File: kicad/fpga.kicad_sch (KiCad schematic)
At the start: 109 parts, among them Q4 BSS138LT1G, U1 XC7A100T-2FGG676I, X4 50MHz CMOS

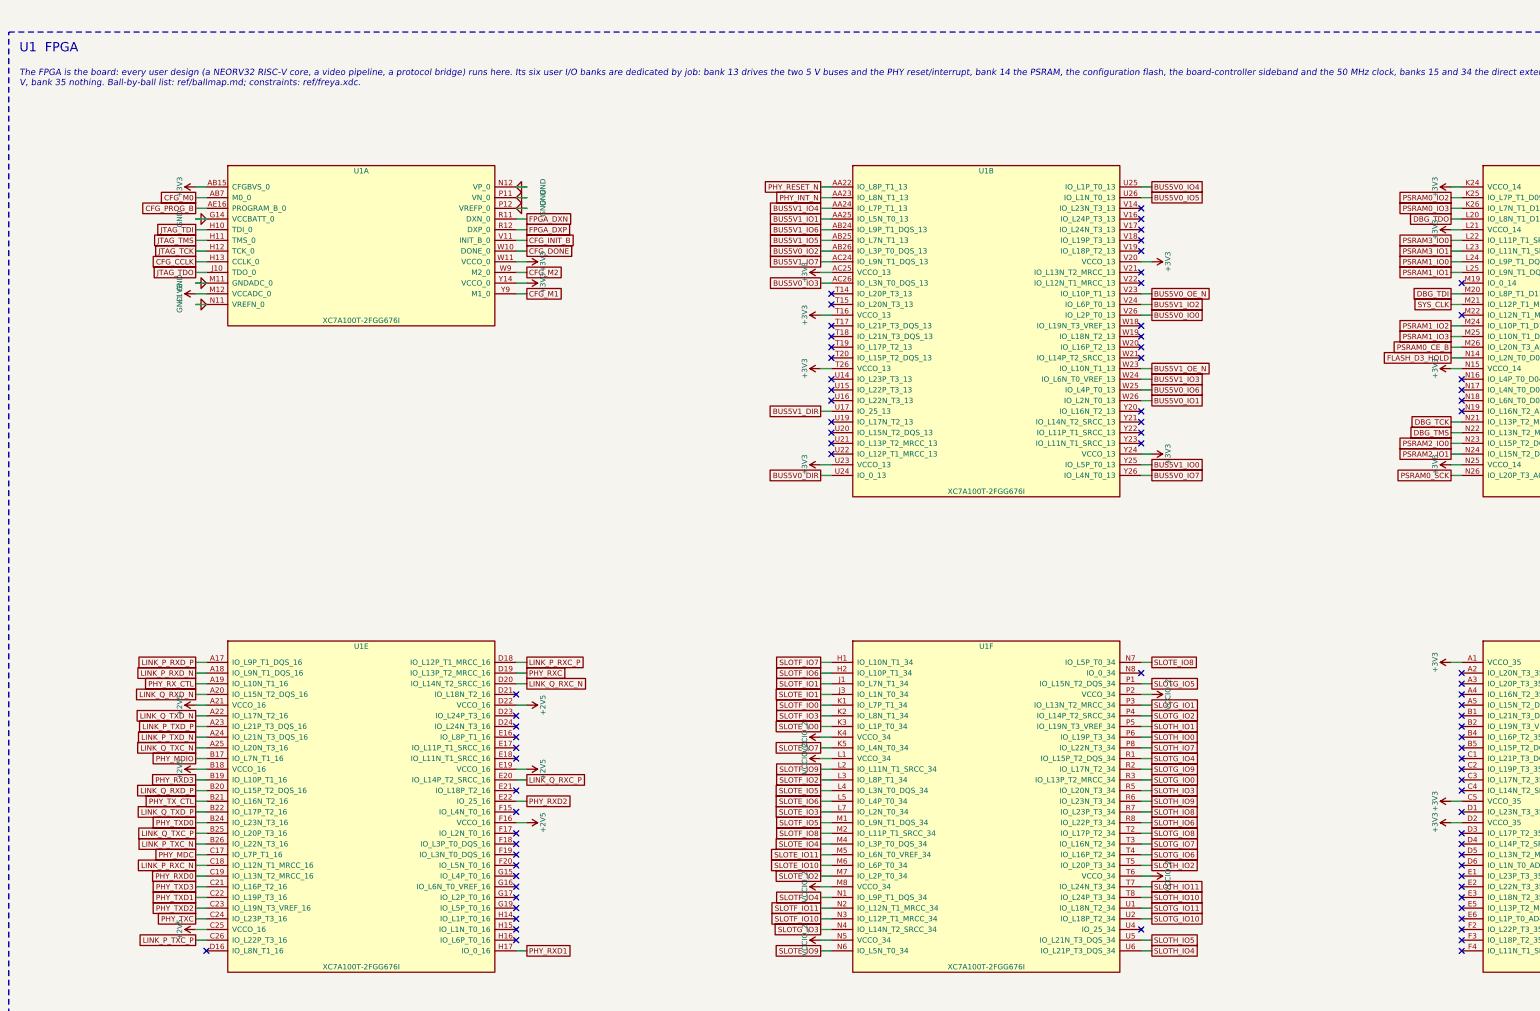
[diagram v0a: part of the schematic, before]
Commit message: Islands, city plan, HDMI out and the eight-layer stackup
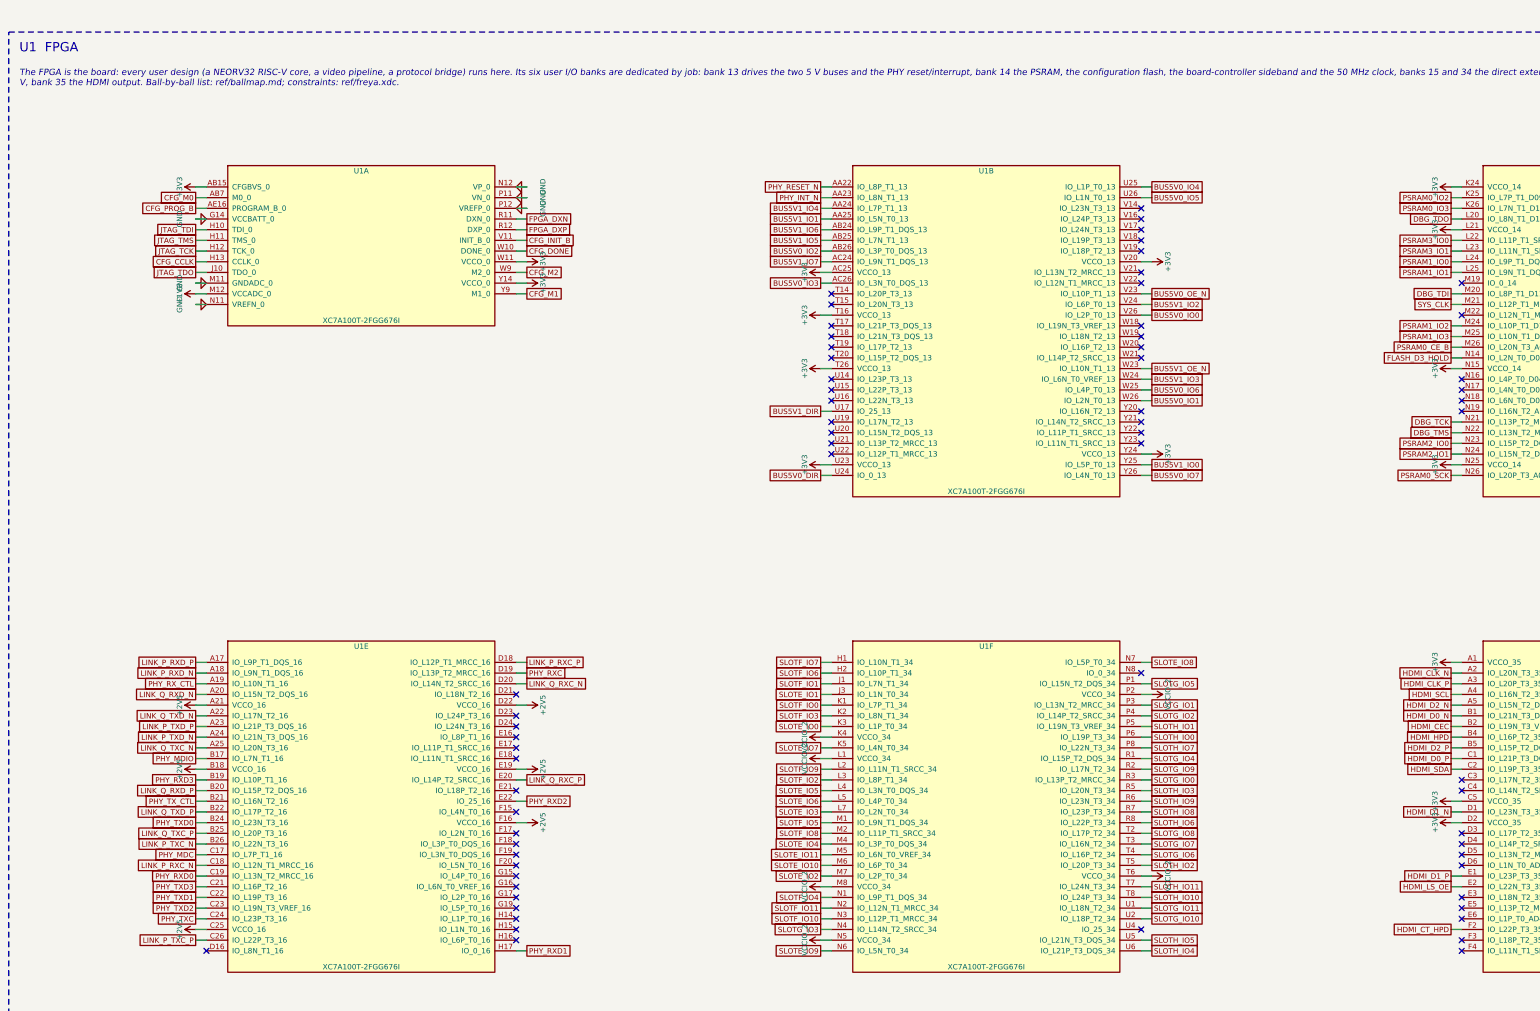
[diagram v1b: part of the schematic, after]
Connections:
- net HDMI_CLK_N: now reaches U1.A2 (IO_L20N_T3_35)
- net HDMI_CLK_P: now reaches U1.A3 (IO_L20P_T3_35)
- net HDMI_SCL: now reaches U1.A4 (IO_L16N_T2_35)
- net HDMI_D2_N: now reaches U1.A5 (IO_L15N_T2_DQS_35)
- net HDMI_D0_N: now reaches U1.B1 (IO_L21N_T3_DQS_35)
- net HDMI_CEC: now reaches U1.B2 (IO_L19N_T3_VREF_35)
- net HDMI_HPD: now reaches U1.B4 (IO_L16P_T2_35)
- net HDMI_D2_P: now reaches U1.B5 (IO_L15P_T2_DQS_35)
- net HDMI_D0_P: now reaches U1.C1 (IO_L21P_T3_DQS_35)
- net HDMI_SDA: now reaches U1.C2 (IO_L19P_T3_35)
- net HDMI_D1_N: now reaches U1.D1 (IO_L23N_T3_35)
- net HDMI_D1_P: now reaches U1.E1 (IO_L23P_T3_35)
- net HDMI_LS_OE: now reaches U1.E2 (IO_L22N_T3_35)
- net HDMI_CT_HPD: now reaches U1.F2 (IO_L22P_T3_35)
- no-connect marks 239 -> 225
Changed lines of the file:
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@@
 	(rectangle (start 30.48 41.91) (end 646.43 521.97) (stroke (width 0.15) (type dash)) (fill (type none)))
 	(text "U1  FPGA" (at 33.02 45.72 0) (effects (font (size 2.2 2.2) (thickness 0.3)) (justify left)))
-	(text "The FPGA is the board: every user design (a NEORV32 RISC-V core, a video pipeline, a protocol bridge) runs here. Its six user I/O banks are dedicated by job: bank 13 drives the two 5 V buses and the PHY reset/interrupt, bank 14 the PSRAM, the configuration flash, the board-controller sideband and the 50 MHz clock, banks 15 and 34 the direct extension slots A-D and E-H at a jumper-selected voltage, bank 16 the network at 2.5\nV, bank 35 nothing. Ball-by-ball list: ref/ballmap.md; constraints: ref/freya.xdc." (at 33.02 50.8 0) (effects (font (size 1.5 1.5) (italic yes)) (justify left top)))
+	(text "The FPGA is the board: every user design (a NEORV32 RISC-V core, a video pipeline, a protocol bridge) runs here. Its six user I/O banks are dedicated by job: bank 13 drives the two 5 V buses and the PHY reset/interrupt, bank 14 the PSRAM, the configuration flash, the board-controller sideband and the 50 MHz clock, banks 15 and 34 the direct extension slots A-D and E-H at a jumper-selected voltage, bank 16 the network at 2.5\nV, bank 35 the HDMI output. Ball-by-ball list: ref/ballmap.md; constraints: ref/freya.xdc." (at 33.02 50.8 0) (effects (font (size 1.5 1.5) (italic yes)) (justify left top)))
 	(rectangle (start 30.48 542.29) (end 543.56 603.25) (stroke (width 0.15) (type dash)) (fill (type none)))
 	(text "decap VCCINT" (at 33.02 546.1 0) (effects (font (size 2.2 2.2) (thickness 0.3)) (justify left)))
@@
 		(instances (project "odin" (path "/c44fb7fe-6133-ad34-68fd-fb66126197ef/8cec9eb4-56b4-e78b-2213-febb3af15411" (reference "#PWR0041") (unit 1))))
 	)
-	(no_connect (at 375.92 194.31))
-	(no_connect (at 375.92 196.85))
-	(no_connect (at 375.92 199.39))
-	(no_connect (at 375.92 201.93))
-	(no_connect (at 375.92 204.47))
-	(no_connect (at 375.92 207.01))
-	(no_connect (at 375.92 209.55))
-	(no_connect (at 375.92 212.09))
-	(no_connect (at 375.92 214.63))
-	(no_connect (at 375.92 217.17))
+	(wire (pts (xy 375.92 194.31) (xy 373.38 194.31)) (stroke (width 0) (type default)))
+	(global_label "HDMI_CLK_N" (shape passive) (at 373.38 194.31 0) (fields_autoplaced yes) (effects (font (size 1.27 1.27)) (justify right)))
+	(wire (pts (xy 375.92 196.85) (xy 373.38 196.85)) (stroke (width 0) (type default)))
+	(global_label "HDMI_CLK_P" (shape passive) (at 373.38 196.85 0) (fields_autoplaced yes) (effects (font (size 1.27 1.27)) (justify right)))
+	(wire (pts (xy 375.92 199.39) (xy 373.38 199.39)) (stroke (width 0) (type default)))
+	(global_label "HDMI_SCL" (shape passive) (at 373.38 199.39 0) (fields_autoplaced yes) (effects (font (size 1.27 1.27)) (justify right)))
+	(wire (pts (xy 375.92 201.93) (xy 373.38 201.93)) (stroke (width 0) (type default)))
+	(global_label "HDMI_D2_N" (shape passive) (at 373.38 201.93 0) (fields_autoplaced yes) (effects (font (size 1.27 1.27)) (justify right)))
+	(wire (pts (xy 375.92 204.47) (xy 373.38 204.47)) (stroke (width 0) (type default)))
+	(global_label "HDMI_D0_N" (shape passive) (at 373.38 204.47 0) (fields_autoplaced yes) (effects (font (size 1.27 1.27)) (justify right)))
+	(wire (pts (xy 375.92 207.01) (xy 373.38 207.01)) (stroke (width 0) (type default)))
+	(global_label "HDMI_CEC" (shape passive) (at 373.38 207.01 0) (fields_autoplaced yes) (effects (font (size 1.27 1.27)) (justify right)))
+	(wire (pts (xy 375.92 209.55) (xy 373.38 209.55)) (stroke (width 0) (type default)))
+	(global_label "HDMI_HPD" (shape passive) (at 373.38 209.55 0) (fields_autoplaced yes) (effects (font (size 1.27 1.27)) (justify right)))
+	(wire (pts (xy 375.92 212.09) (xy 373.38 212.09)) (stroke (width 0) (type default)))
+	(global_label "HDMI_D2_P" (shape passive) (at 373.38 212.09 0) (fields_autoplaced yes) (effects (font (size 1.27 1.27)) (justify right)))
+	(wire (pts (xy 375.92 214.63) (xy 373.38 214.63)) (stroke (width 0) (type default)))
+	(global_label "HDMI_D0_P" (shape passive) (at 373.38 214.63 0) (fields_autoplaced yes) (effects (font (size 1.27 1.27)) (justify right)))
+	(wire (pts (xy 375.92 217.17) (xy 373.38 217.17)) (stroke (width 0) (type default)))
+	(global_label "HDMI_SDA" (shape passive) (at 373.38 217.17 0) (fields_autoplaced yes) (effects (font (size 1.27 1.27)) (justify right)))
 	(no_connect (at 375.92 219.71))
 	(no_connect (at 375.92 222.25))
@@
 		(instances (project "odin" (path "/c44fb7fe-6133-ad34-68fd-fb66126197ef/8cec9eb4-56b4-e78b-2213-febb3af15411" (reference "#PWR0042") (unit 1))))
 	)
-	(no_connect (at 375.92 227.33))
+	(wire (pts (xy 375.92 227.33) (xy 373.38 227.33)) (stroke (width 0) (type default)))
+	(global_label "HDMI_D1_N" (shape passive) (at 373.38 227.33 0) (fields_autoplaced yes) (effects (font (size 1.27 1.27)) (justify right)))
 	(wire (pts (xy 375.92 229.87) (xy 373.38 229.87)) (stroke (width 0) (type default)))
 	(symbol (lib_id "power:+3V3") (at 373.38 229.87 90) (unit 1)
@@
 	(no_connect (at 375.92 237.49))
 	(no_connect (at 375.92 240.03))
-	(no_connect (at 375.92 242.57))
-	(no_connect (at 375.92 245.11))
+	(wire (pts (xy 375.92 242.57) (xy 373.38 242.57)) (stroke (width 0) (type default)))
+	(global_label "HDMI_D1_P" (shape passive) (at 373.38 242.57 0) (fields_autoplaced yes) (effects (font (size 1.27 1.27)) (justify right)))
+	(wire (pts (xy 375.92 245.11) (xy 373.38 245.11)) (stroke (width 0) (type default)))
+	(global_label "HDMI_LS_OE" (shape passive) (at 373.38 245.11 0) (fields_autoplaced yes) (effects (font (size 1.27 1.27)) (justify right)))
 	(no_connect (at 375.92 247.65))
 	(no_connect (at 375.92 250.19))
 	(no_connect (at 375.92 252.73))
-	(no_connect (at 375.92 255.27))
+	(wire (pts (xy 375.92 255.27) (xy 373.38 255.27)) (stroke (width 0) (type default)))
+	(global_label "HDMI_CT_HPD" (shape passive) (at 373.38 255.27 0) (fields_autoplaced yes) (effects (font (size 1.27 1.27)) (justify right)))
 	(no_connect (at 375.92 257.81))
 	(no_connect (at 375.92 260.35))
